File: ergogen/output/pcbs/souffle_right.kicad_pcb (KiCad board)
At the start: 2 copper layers, 130 x 99.4 mm, 60 parts

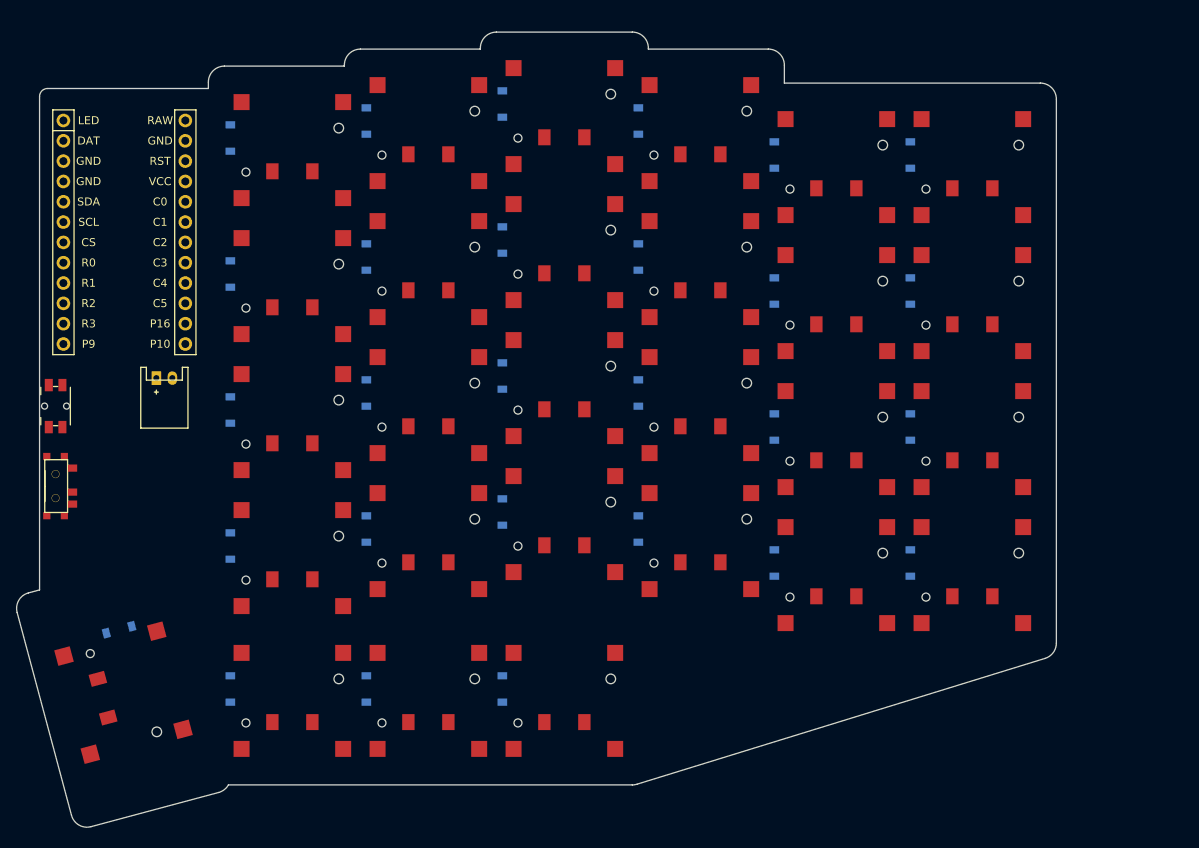
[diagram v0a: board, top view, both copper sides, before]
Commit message: feat: choc version
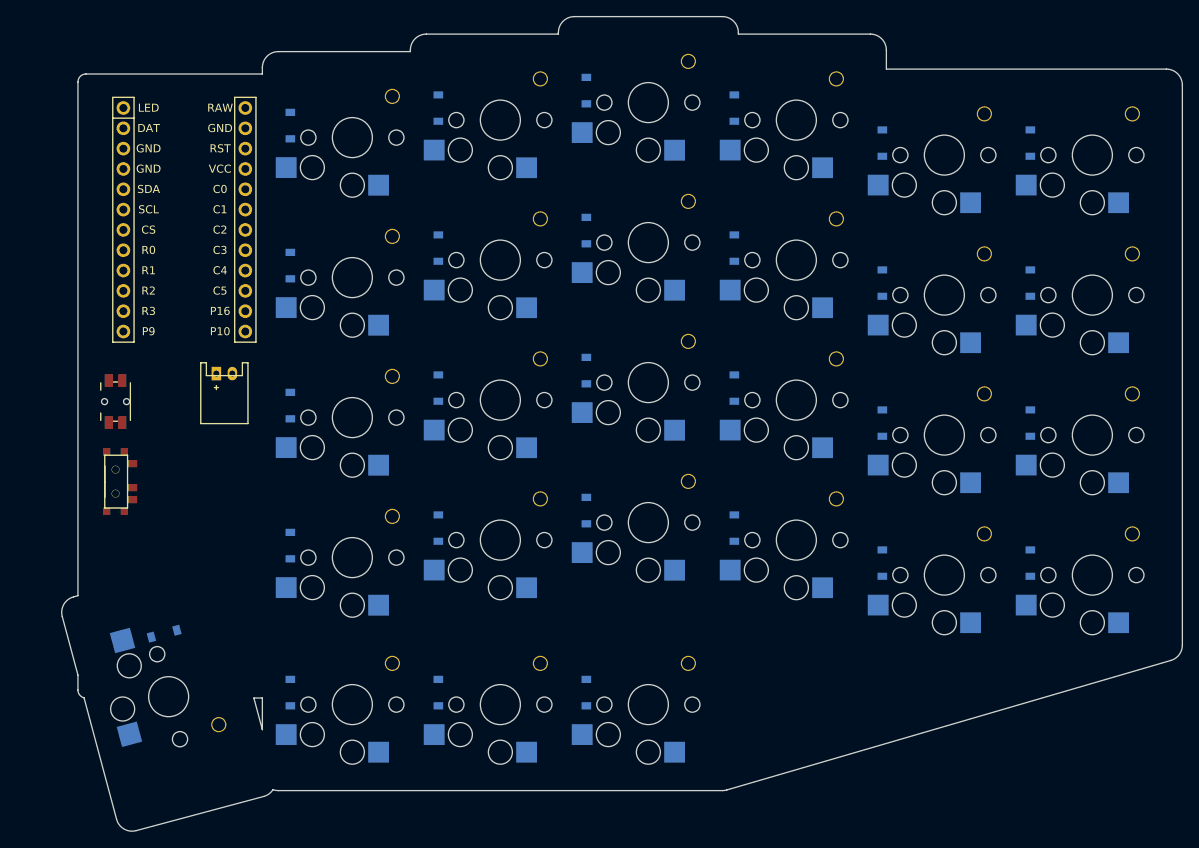
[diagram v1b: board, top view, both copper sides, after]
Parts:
- S1, S10, S11, S12, S13, S14, S15, S16, S17, S18, S19, S2, S20, S21, S22, S23, S24, S25, S26, S27, S28, S3, S4, S5, S6, S7, S8, S9: footprint CPG1316S01D02_mikeholscher -> ceoloide:switch_choc_v1_v2; moved to B.Cu
- moved D4 15.1 mm to (357.2, 46.0), turned to 90 degrees
- moved S4 15.1 mm to (365.0, 47.5), turned to -180 degrees
- moved D3 15.0 mm to (357.2, 63.5), turned to 90 degrees
- moved S3 15.0 mm to (365.0, 65.0), turned to -180 degrees
- moved D2 15.0 mm to (357.2, 81.0), turned to 90 degrees
- moved S2 15.0 mm to (365.0, 82.5), turned to -180 degrees
- moved D1 15.0 mm to (357.2, 98.5), turned to 90 degrees
- moved S1 15.0 mm to (365.0, 100.0), turned to -180 degrees
- moved D8 13.6 mm to (338.8, 46.0), turned to 90 degrees
- moved S8 13.6 mm to (346.5, 47.5), turned to -180 degrees
- moved D7 13.5 mm to (338.8, 63.5), turned to 90 degrees
- moved S7 13.5 mm to (346.5, 65.0), turned to -180 degrees
- moved D6 13.5 mm to (338.8, 81.0), turned to 90 degrees
- moved S6 13.5 mm to (346.5, 82.5), turned to -180 degrees
- moved D5 13.5 mm to (338.8, 98.5), turned to 90 degrees
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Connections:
- S1 pad 1: mirror_outer_bottom -> C0
- S1 pad 2: C0 -> mirror_outer_bottom
- S10 pad 1: mirror_ring_home -> C2
- S10 pad 2: C2 -> mirror_ring_home
- S11 pad 1: mirror_ring_top -> C2
- S11 pad 2: C2 -> mirror_ring_top
- S12 pad 1: mirror_ring_number -> C2
- S12 pad 2: C2 -> mirror_ring_number
- S13 pad 1: mirror_middle_bottom -> C3
- S13 pad 2: C3 -> mirror_middle_bottom
- S14 pad 1: mirror_middle_home -> C3
- S14 pad 2: C3 -> mirror_middle_home
- S15 pad 1: mirror_middle_top -> C3
- S15 pad 2: C3 -> mirror_middle_top
- S16 pad 1: mirror_middle_number -> C3
- S16 pad 2: C3 -> mirror_middle_number
- S17 pad 1: mirror_index_bottom -> C4
- S17 pad 2: C4 -> mirror_index_bottom
- S18 pad 1: mirror_index_home -> C4
- S18 pad 2: C4 -> mirror_index_home
- S19 pad 1: mirror_index_top -> C4
- S19 pad 2: C4 -> mirror_index_top
- S2 pad 1: mirror_outer_home -> C0
- S2 pad 2: C0 -> mirror_outer_home
- S20 pad 1: mirror_index_number -> C4
- S20 pad 2: C4 -> mirror_index_number
- S21 pad 1: mirror_inner_bottom -> C5
- S21 pad 2: C5 -> mirror_inner_bottom
- S22 pad 1: mirror_inner_home -> C5
- S22 pad 2: C5 -> mirror_inner_home
- S23 pad 1: mirror_inner_top -> C5
- S23 pad 2: C5 -> mirror_inner_top
- S24 pad 1: mirror_inner_number -> C5
- S24 pad 2: C5 -> mirror_inner_number
- S25 pad 1: mirror_inward_home -> C2
- S25 pad 2: C2 -> mirror_inward_home
- S26 pad 1: mirror_outward_home -> C3
- S26 pad 2: C3 -> mirror_outward_home
- S27 pad 1: mirror_small_thumbkey_home -> C4
- S27 pad 2: C4 -> mirror_small_thumbkey_home
- S28 pad 1: mirror_thumbkey_home -> C5
- S28 pad 2: C5 -> mirror_thumbkey_home
- S3 pad 1: mirror_outer_top -> C0
- S3 pad 2: C0 -> mirror_outer_top
- S4 pad 1: mirror_outer_number -> C0
- S4 pad 2: C0 -> mirror_outer_number
- S5 pad 1: mirror_pinky_bottom -> C1
- S5 pad 2: C1 -> mirror_pinky_bottom
- S6 pad 1: mirror_pinky_home -> C1
- S6 pad 2: C1 -> mirror_pinky_home
- S7 pad 1: mirror_pinky_top -> C1
- S7 pad 2: C1 -> mirror_pinky_top
- S8 pad 1: mirror_pinky_number -> C1
- S8 pad 2: C1 -> mirror_pinky_number
- S9 pad 1: mirror_ring_bottom -> C2
- S9 pad 2: C2 -> mirror_ring_bottom
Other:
- board size 130 x 99.4 mm -> 140.1 x 101.8 mm
